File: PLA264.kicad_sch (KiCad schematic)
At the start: 10 parts, among them J1 PLA_Socket, U1 GAL16V8

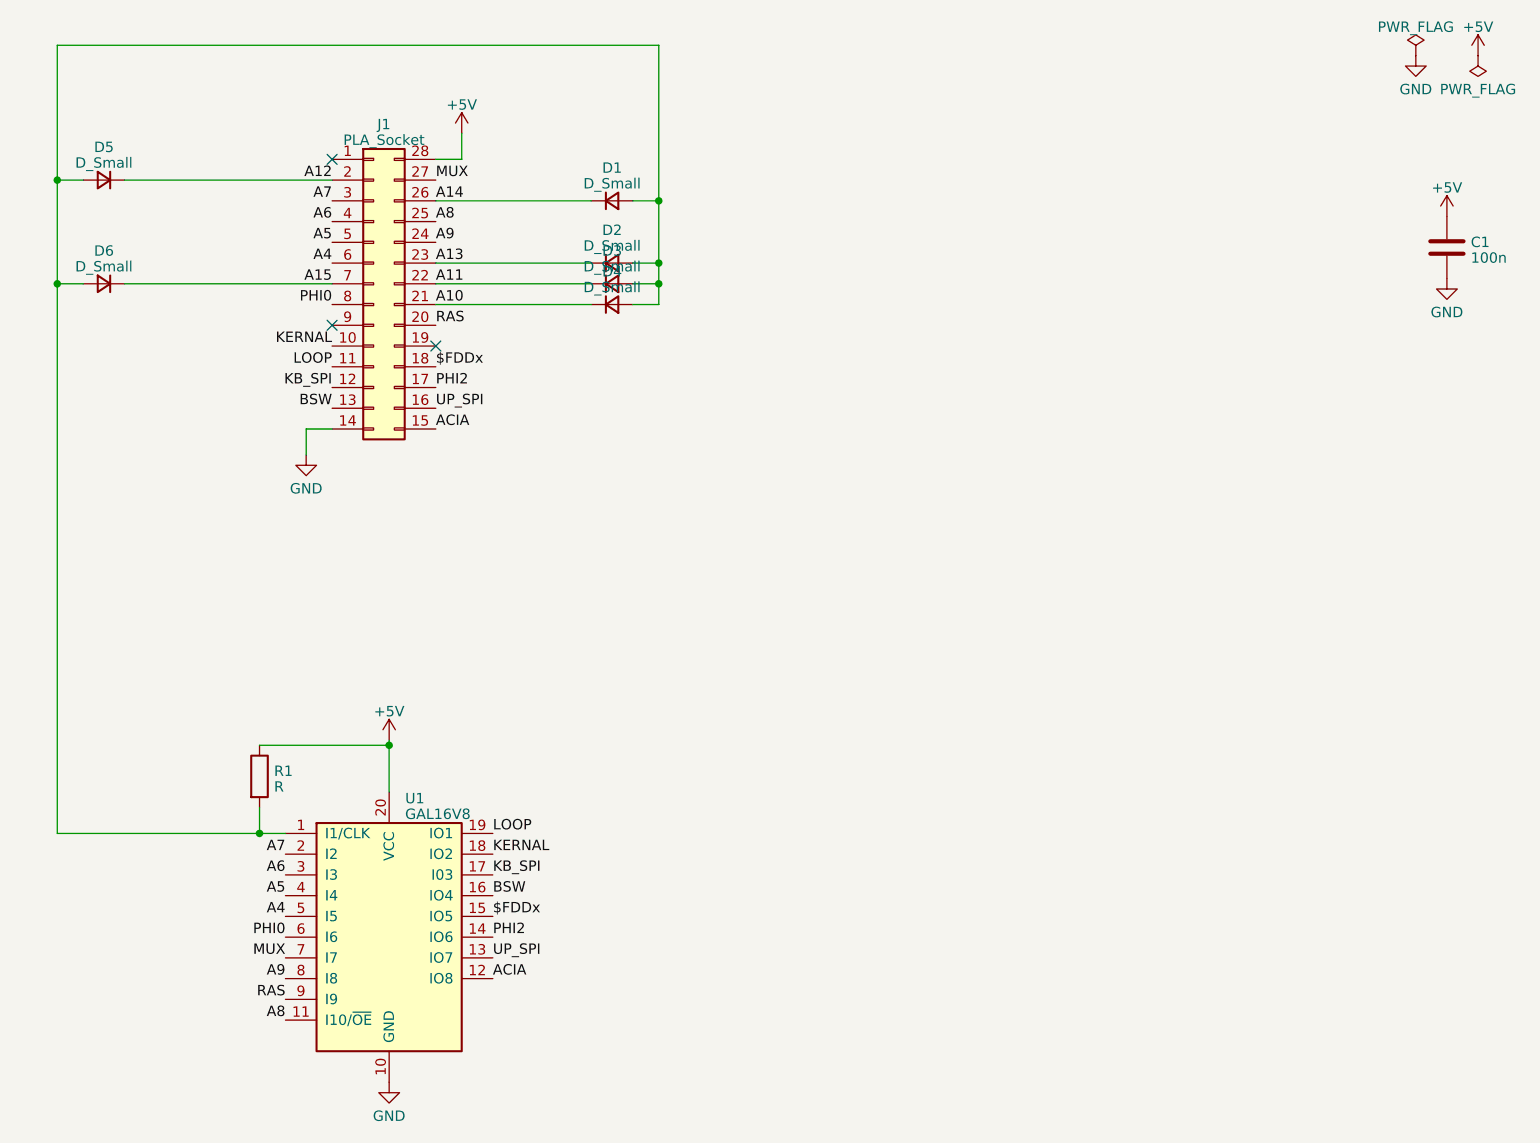
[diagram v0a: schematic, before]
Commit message: Cleaning up.
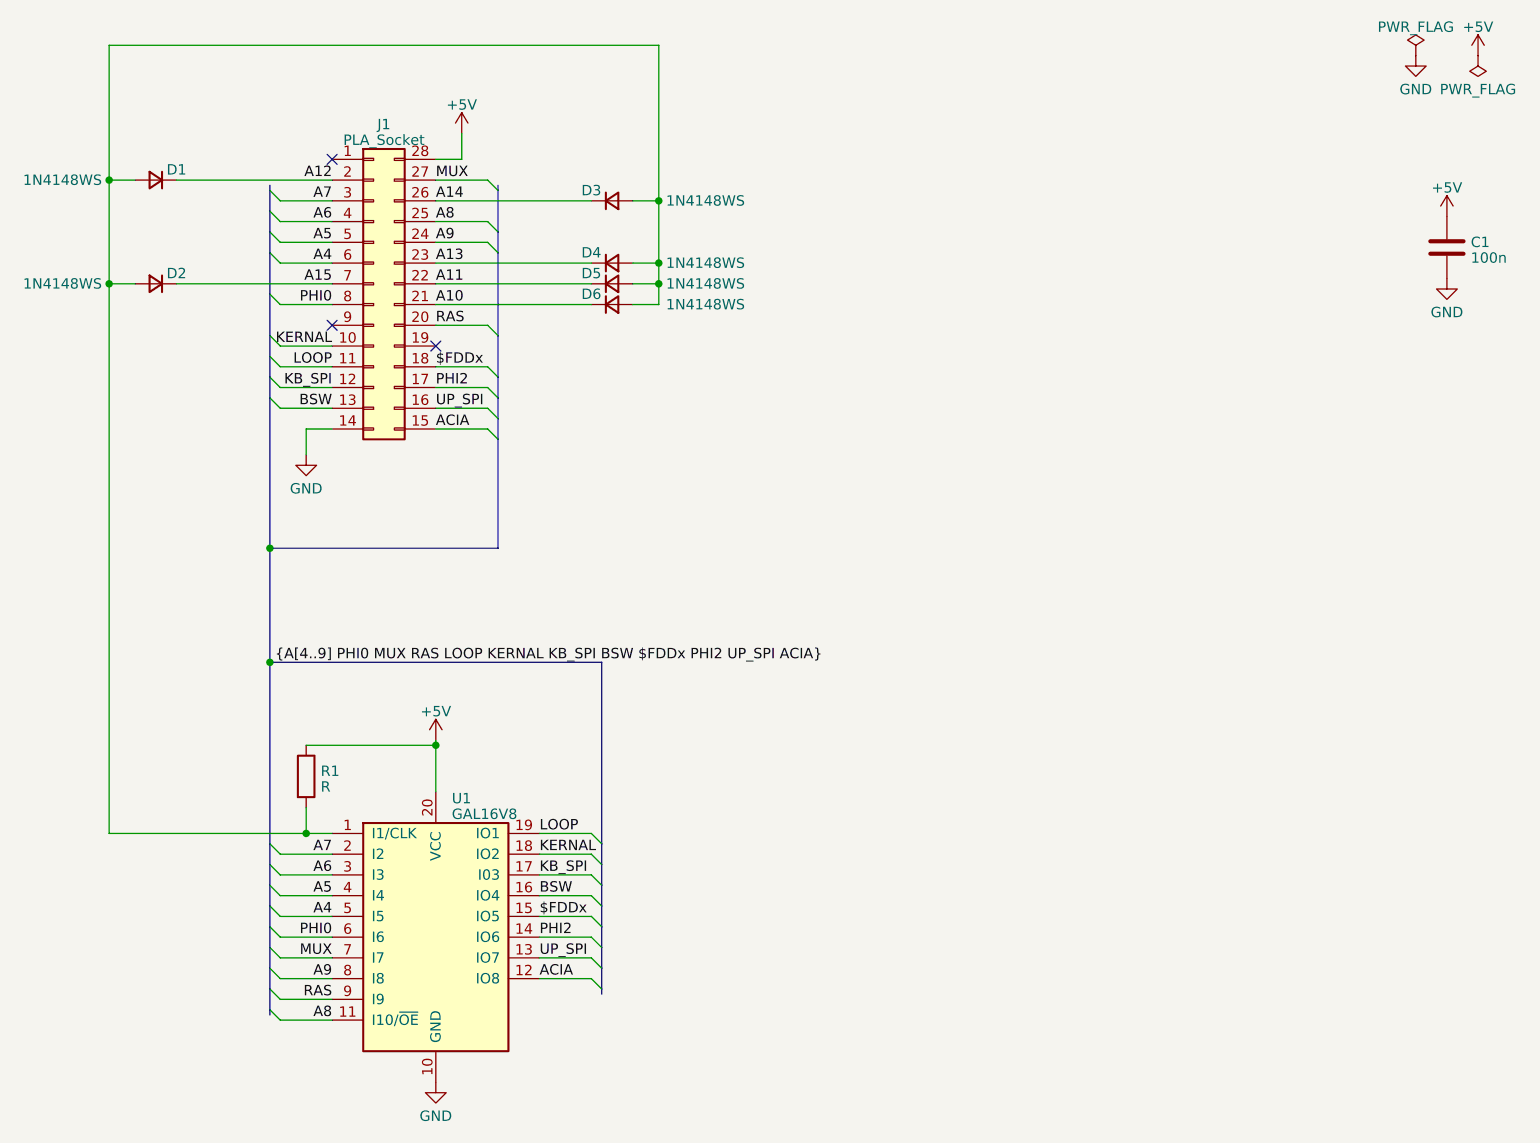
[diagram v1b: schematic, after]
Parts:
- D1: renamed from D5; value D_Small -> 1N4148WS
- D2: renamed from D6; value D_Small -> 1N4148WS
- D3: renamed from D1; value D_Small -> 1N4148WS
- D4: renamed from D2; value D_Small -> 1N4148WS
- D5: renamed from D3; value D_Small -> 1N4148WS
- D6: renamed from D4; value D_Small -> 1N4148WS
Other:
- company: (none) -> www.hackup.net
- title: (none) -> PLA264
- moved on the sheet: D1, D2, R1, U1
